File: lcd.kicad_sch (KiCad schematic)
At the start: 7 parts, among them J2 LCD 3.2" 240x320 Conn_01x14_P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, Q4 SI2301CDS-T1-GE3

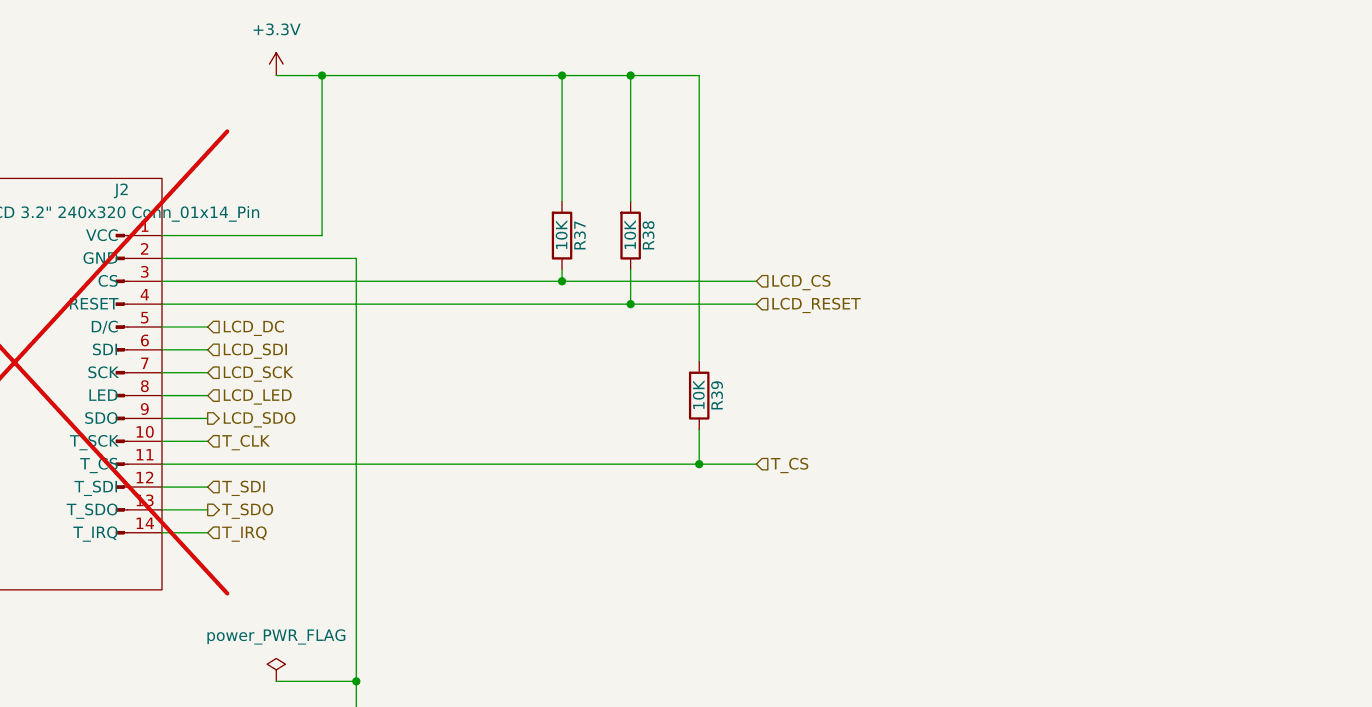
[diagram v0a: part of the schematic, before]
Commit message: version 2 changes
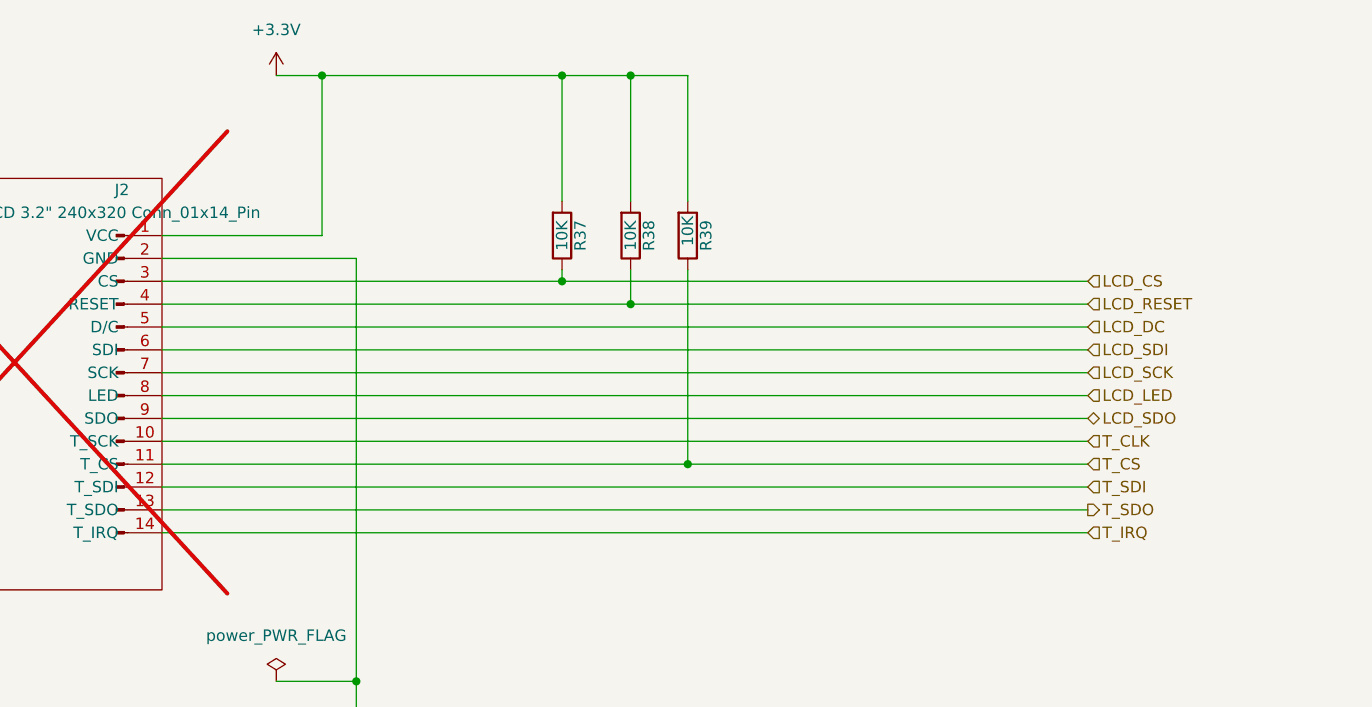
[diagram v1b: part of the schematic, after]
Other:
- moved on the sheet: R39
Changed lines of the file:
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@@
 	)
 	(junction
-		(at 195.58 71.12)
+		(at 194.31 71.12)
 		(diameter 0)
 		(color 0 0 0 0)
@@
 	(wire
 		(pts
-			(xy 135.89 60.96) (xy 140.97 60.96)
+			(xy 135.89 60.96) (xy 238.76 60.96)
 		)
 		(stroke
@@
 	(wire
 		(pts
-			(xy 135.89 71.12) (xy 195.58 71.12)
-		)
-		(stroke
-			(width 0)
-			(type default)
-		)
-	)
-	(wire
-		(pts
-			(xy 135.89 58.42) (xy 140.97 58.42)
+			(xy 135.89 71.12) (xy 194.31 71.12)
+		)
+		(stroke
+			(width 0)
+			(type default)
+		)
+	)
+	(wire
+		(pts
+			(xy 135.89 58.42) (xy 238.76 58.42)
 		)
 		(stroke
@@
 	(wire
 		(pts
-			(xy 180.34 50.8) (xy 201.93 50.8)
+			(xy 180.34 50.8) (xy 238.76 50.8)
 		)
 		(stroke
@@
 	(wire
 		(pts
-			(xy 195.58 67.31) (xy 195.58 71.12)
-		)
-		(stroke
-			(width 0)
-			(type default)
-		)
-	)
-	(wire
-		(pts
-			(xy 135.89 66.04) (xy 140.97 66.04)
-		)
-		(stroke
-			(width 0)
-			(type default)
-		)
-	)
-	(wire
-		(pts
-			(xy 135.89 78.74) (xy 140.97 78.74)
-		)
-		(stroke
-			(width 0)
-			(type default)
-		)
-	)
-	(wire
-		(pts
-			(xy 135.89 55.88) (xy 140.97 55.88)
+			(xy 194.31 49.53) (xy 194.31 71.12)
+		)
+		(stroke
+			(width 0)
+			(type default)
+		)
+	)
+	(wire
+		(pts
+			(xy 135.89 66.04) (xy 238.76 66.04)
+		)
+		(stroke
+			(width 0)
+			(type default)
+		)
+	)
+	(wire
+		(pts
+			(xy 135.89 78.74) (xy 238.76 78.74)
+		)
+		(stroke
+			(width 0)
+			(type default)
+		)
+	)
+	(wire
+		(pts
+			(xy 135.89 55.88) (xy 238.76 55.88)
 		)
 		(stroke
@@
 	(wire
 		(pts
-			(xy 135.89 73.66) (xy 140.97 73.66)
-		)
-		(stroke
-			(width 0)
-			(type default)
-		)
-	)
-	(wire
-		(pts
-			(xy 135.89 76.2) (xy 140.97 76.2)
+			(xy 135.89 73.66) (xy 238.76 73.66)
+		)
+		(stroke
+			(width 0)
+			(type default)
+		)
+	)
+	(wire
+		(pts
+			(xy 135.89 76.2) (xy 238.76 76.2)
 		)
 		(stroke
@@
 	(wire
 		(pts
-			(xy 135.89 63.5) (xy 140.97 63.5)
+			(xy 194.31 71.12) (xy 238.76 71.12)
+		)
+		(stroke
+			(width 0)
+			(type default)
+		)
+	)
+	(wire
+		(pts
+			(xy 135.89 63.5) (xy 238.76 63.5)
 		)
 		(stroke
@@
 	(wire
 		(pts
-			(xy 195.58 59.69) (xy 195.58 27.94)
-		)
-		(stroke
-			(width 0)
-			(type default)
-		)
-	)
-	(wire
-		(pts
-			(xy 195.58 27.94) (xy 187.96 27.94)
-		)
-		(stroke
-			(width 0)
-			(type default)
-		)
-	)
-	(wire
-		(pts
-			(xy 187.96 53.34) (xy 201.93 53.34)
-		)
-		(stroke
-			(width 0)
-			(type default)
-		)
-	)
-	(wire
-		(pts
-			(xy 195.58 71.12) (xy 201.93 71.12)
+			(xy 194.31 41.91) (xy 194.31 27.94)
+		)
+		(stroke
+			(width 0)
+			(type default)
+		)
+	)
+	(wire
+		(pts
+			(xy 194.31 27.94) (xy 187.96 27.94)
+		)
+		(stroke
+			(width 0)
+			(type default)
+		)
+	)
+	(wire
+		(pts
+			(xy 187.96 53.34) (xy 238.76 53.34)
 		)
 		(stroke
@@
 	(wire
 		(pts
-			(xy 135.89 68.58) (xy 140.97 68.58)
+			(xy 135.89 68.58) (xy 238.76 68.58)
 		)
 		(stroke
@@
 	(hierarchical_label "LCD_SDI"
 		(shape input)
-		(at 140.97 58.42 0)
+		(at 238.76 58.42 0)
 		(fields_autoplaced yes)
 		(effects
@@
 	(hierarchical_label "LCD_LED"
 		(shape input)
-		(at 140.97 63.5 0)
+		(at 238.76 63.5 0)
 		(fields_autoplaced yes)
 		(effects
@@
 	(hierarchical_label "T_CS"
 		(shape input)
-		(at 201.93 71.12 0)
+		(at 238.76 71.12 0)
 		(fields_autoplaced yes)
 		(effects
@@
 	(hierarchical_label "T_IRQ"
 		(shape input)
-		(at 140.97 78.74 0)
+		(at 238.76 78.74 0)
 		(fields_autoplaced yes)
 		(effects
@@
 	(hierarchical_label "T_SDI"
 		(shape input)
-		(at 140.97 73.66 0)
+		(at 238.76 73.66 0)
 		(fields_autoplaced yes)
 		(effects
@@
 	(hierarchical_label "T_SDO"
 		(shape output)
-		(at 140.97 76.2 0)
+		(at 238.76 76.2 0)
 		(fields_autoplaced yes)
 		(effects
@@
 	(hierarchical_label "LCD_DC"
 		(shape input)
-		(at 140.97 55.88 0)
+		(at 238.76 55.88 0)
 		(fields_autoplaced yes)
 		(effects
@@
 	(hierarchical_label "T_CLK"
 		(shape input)
-		(at 140.97 68.58 0)
+		(at 238.76 68.58 0)
 		(fields_autoplaced yes)
 		(effects
@@
 	)
 	(hierarchical_label "LCD_SDO"
-		(shape output)
-		(at 140.97 66.04 0)
+		(shape tri_state)
+		(at 238.76 66.04 0)
 		(fields_autoplaced yes)
 		(effects
@@
 	(hierarchical_label "LCD_SCK"
 		(shape input)
-		(at 140.97 60.96 0)
+		(at 238.76 60.96 0)
 		(fields_autoplaced yes)
 		(effects
@@
 	(hierarchical_label "LCD_RESET"
 		(shape input)
-		(at 201.93 53.34 0)
+		(at 238.76 53.34 0)
 		(fields_autoplaced yes)
 		(effects
@@
 	(hierarchical_label "LCD_CS"
 		(shape input)
-		(at 201.93 50.8 0)
+		(at 238.76 50.8 0)
 		(fields_autoplaced yes)
 		(effects
@@
 	)
 	(symbol
-		(lib_id "l8-kicad-rescue:GND-power")
+		(lib_id "power:GND")
 		(at 157.48 118.11 0)
 		(unit 1)
@@
 	(symbol
 		(lib_id "Device:R")
-		(at 195.58 63.5 0)
+		(at 194.31 45.72 0)
 		(mirror x)
 		(unit 1)
@@
 		(dnp no)
 		(property "Reference" "R39"
-			(at 197.612 63.5 90)
+			(at 196.342 45.72 90)
 			(effects
 				(font
@@
 		)
 		(property "Value" "10K"
-			(at 195.58 63.5 90)
+			(at 194.31 45.212 90)
 			(effects
 				(font
@@
 		)
 		(property "Footprint" "Resistor_SMD:R_0603_1608Metric"
-			(at 254.762 121.92 90)
+			(at 253.492 104.14 90)
 			(effects
 				(font
@@
 		)
 		(property "Datasheet" "~"
-			(at 344.17 122.555 0)
+			(at 342.9 104.775 0)
 			(effects
 				(font
@@
 		)
 		(property "Description" "Resistor"
-			(at 195.58 63.5 0)
+			(at 194.31 45.72 0)
 			(effects
 				(font
@@
 		)
 		(property "Part #" ""
-			(at 77.47 -43.18 0)
+			(at 76.2 -60.96 0)
 			(effects
 				(font
@@
 		)
 		(property "VEND" ""
-			(at 77.47 -43.18 0)
+			(at 76.2 -60.96 0)
 			(effects
 				(font
@@
 		)
 		(property "VEND#" ""
-			(at 77.47 -43.18 0)
+			(at 76.2 -60.96 0)
 			(effects
 				(font
@@
 		)
 		(property "Manufacturer" ""
-			(at 77.47 -43.18 0)
+			(at 76.2 -60.96 0)
 			(effects
 				(font
@@
 		)
 		(property "LCSC" "C25804"
-			(at 195.58 63.5 0)
+			(at 194.31 45.72 0)
 			(effects
 				(font
@@
 		)
 		(property "Sim.Device" ""
-			(at 195.58 63.5 0)
+			(at 194.31 45.72 0)
 			(effects
 				(font
@@
 		)
 		(property "Sim.Pins" ""
-			(at 195.58 63.5 0)
+			(at 194.31 45.72 0)
 			(effects
 				(font
@@
 		)
 		(property "Silkscreen" ""
-			(at 195.58 63.5 0)
+			(at 194.31 45.72 0)
 			(effects
 				(font
@@
 	)
 	(symbol
-		(lib_id "l8-kicad-rescue:GND-power")
+		(lib_id "power:GND")
 		(at 134.62 119.38 0)
 		(unit 1)
@@
 	)
 	(symbol
-		(lib_id "l8-kicad-rescue:PWR_FLAG-power")
+		(lib_id "power:PWR_FLAG")
 		(at 148.59 95.25 0)
 		(unit 1)
@@
 			)
 		)
-		(property "Datasheet" ""
+		(property "Datasheet" "~"
 			(at 148.59 95.25 0)
 			(effects
@@
 			)
 		)
-		(property "Description" ""
+		(property "Description" "Special symbol for telling ERC where power comes from"
 			(at 148.59 95.25 0)
 			(effects
